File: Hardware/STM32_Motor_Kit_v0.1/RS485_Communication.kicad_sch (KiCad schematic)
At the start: 23 parts, among them J7 Conn_01x02_Male, U14 THVD1500D

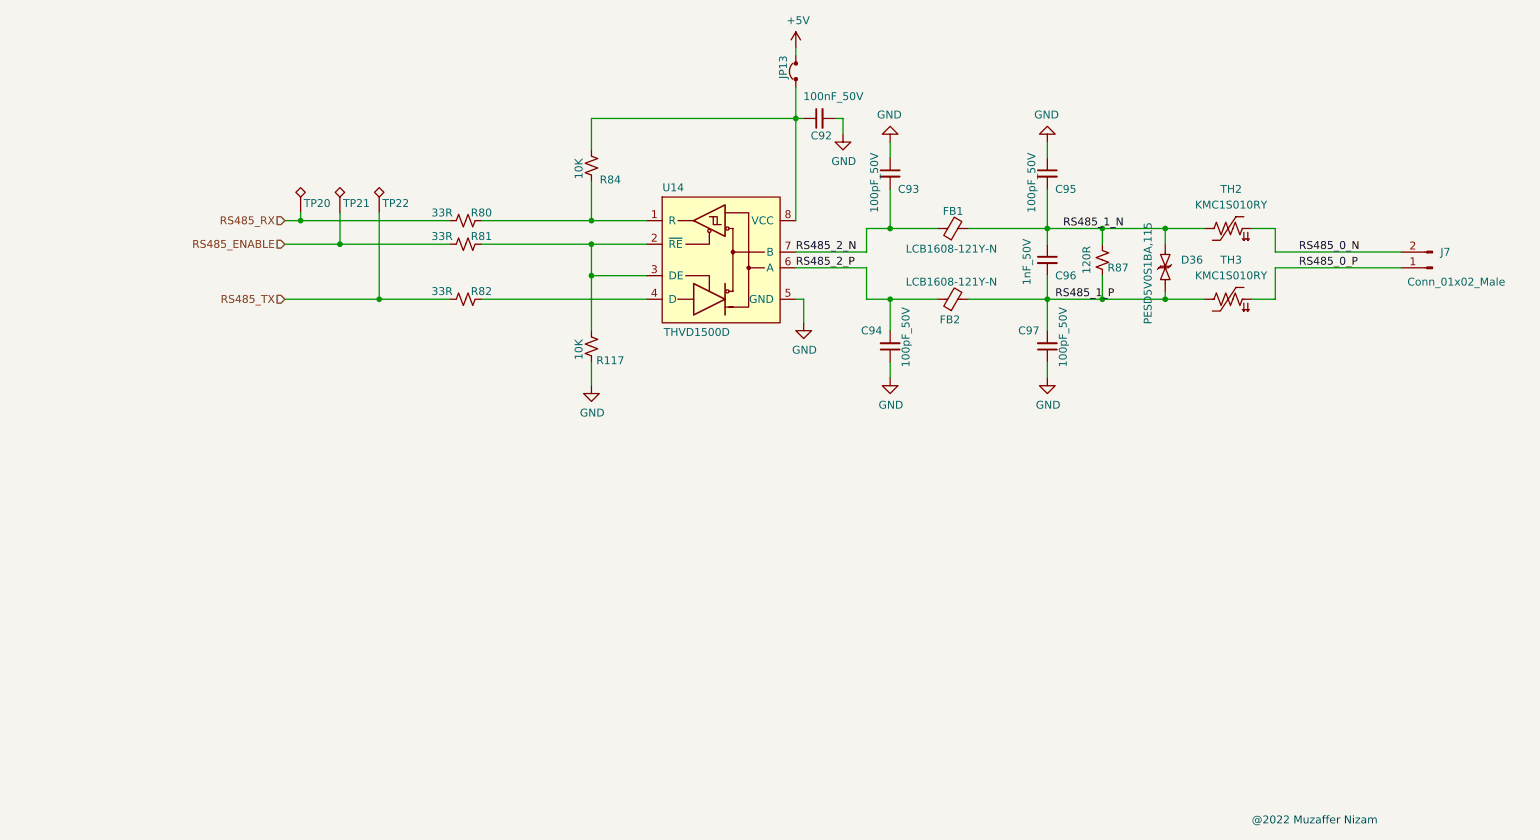
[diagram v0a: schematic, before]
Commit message: 12.01.2025
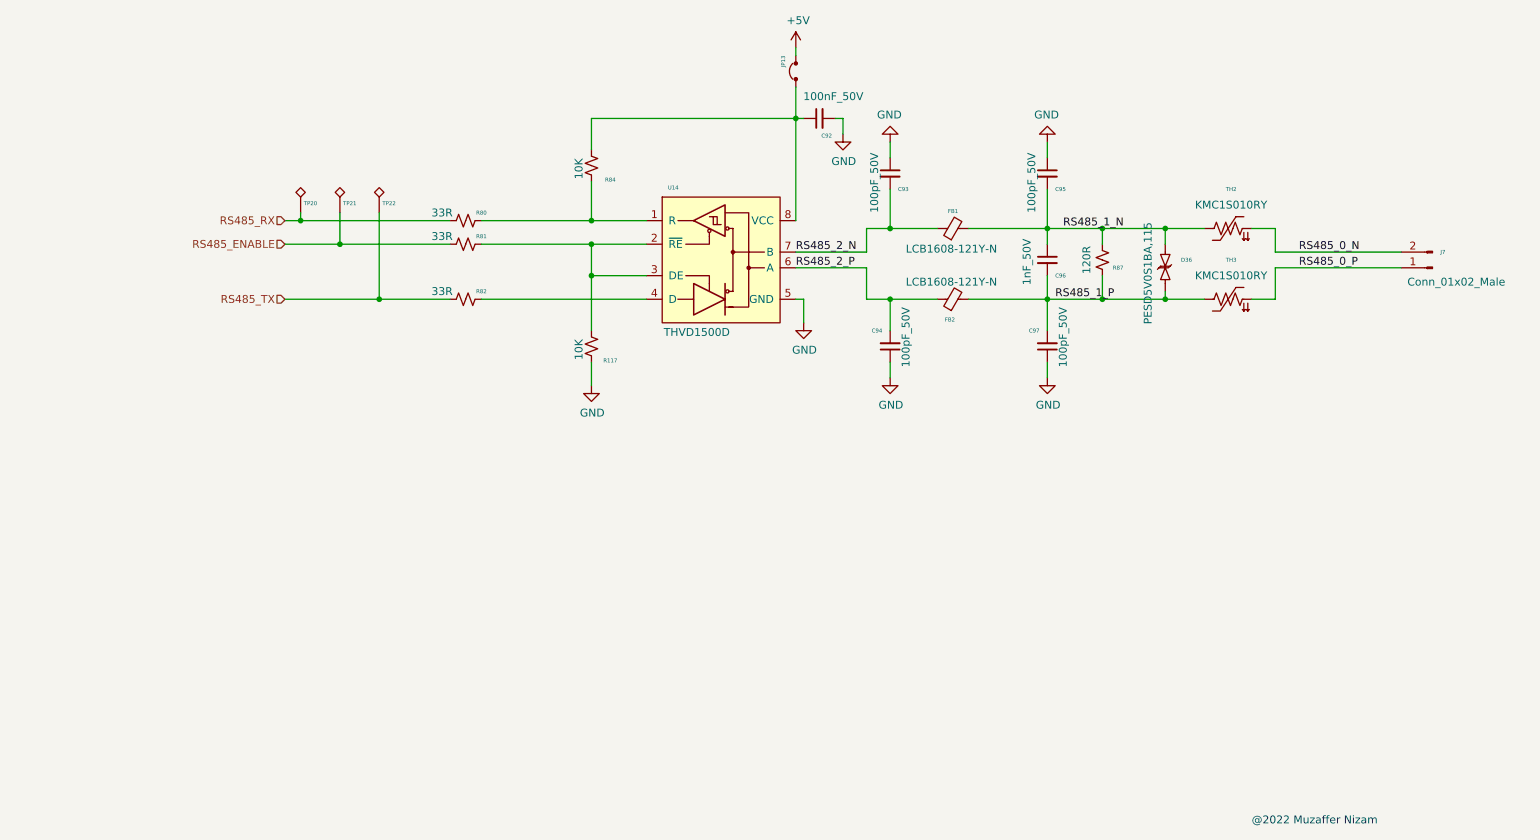
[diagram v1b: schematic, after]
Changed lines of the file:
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@@
 			(effects
 				(font
-					(size 1.27 1.27)
+					(face "Arial")
+					(size 0.635 0.635)
 				)
 			)
@@
 			(effects
 				(font
-					(size 1.27 1.27)
+					(face "Arial")
+					(size 0.635 0.635)
 				)
 				(justify left)
@@
 			(effects
 				(font
-					(size 1.27 1.27)
+					(face "Arial")
+					(size 0.635 0.635)
 				)
 			)
@@
 			(effects
 				(font
-					(size 1.27 1.27)
+					(face "Arial")
+					(size 0.635 0.635)
 				)
 				(justify right)
@@
 			(effects
 				(font
-					(size 1.27 1.27)
+					(face "Arial")
+					(size 0.635 0.635)
 				)
 				(justify left)
@@
 			(effects
 				(font
-					(size 1.27 1.27)
+					(face "Arial")
+					(size 0.635 0.635)
 				)
 			)
@@
 			(effects
 				(font
-					(size 1.27 1.27)
+					(face "Arial")
+					(size 0.635 0.635)
 				)
 				(justify left)
@@
 			(effects
 				(font
-					(size 1.27 1.27)
+					(face "Arial")
+					(size 0.635 0.635)
 				)
 			)
@@
 			(effects
 				(font
-					(size 1.27 1.27)
+					(face "Arial")
+					(size 0.635 0.635)
 				)
 			)
@@
 			(effects
 				(font
-					(size 1.27 1.27)
+					(face "Arial")
+					(size 0.635 0.635)
 				)
 				(justify left)
@@
 			(effects
 				(font
-					(size 1.27 1.27)
+					(face "Arial")
+					(size 0.635 0.635)
 				)
 				(hide yes)
@@
 			(effects
 				(font
-					(size 1.27 1.27)
+					(face "Arial")
+					(size 0.635 0.635)
 				)
 				(hide yes)
@@
 			(effects
 				(font
-					(size 1.27 1.27)
+					(face "Arial")
+					(size 0.635 0.635)
 				)
 				(justify left)
@@
 			(effects
 				(font
-					(size 1.27 1.27)
+					(face "Arial")
+					(size 0.635 0.635)
 				)
 			)
@@
 			(effects
 				(font
-					(size 1.27 1.27)
+					(face "Arial")
+					(size 0.635 0.635)
 				)
 				(justify right)
@@
 			(effects
 				(font
-					(size 1.27 1.27)
+					(face "Arial")
+					(size 0.635 0.635)
 				)
 				(hide yes)
@@
 			(effects
 				(font
-					(size 1.27 1.27)
+					(face "Arial")
+					(size 0.635 0.635)
 				)
 				(hide yes)
@@
 			(effects
 				(font
-					(size 1.27 1.27)
+					(face "Arial")
+					(size 0.635 0.635)
 				)
 			)
@@
 			(effects
 				(font
-					(size 1.27 1.27)
+					(face "Arial")
+					(size 0.635 0.635)
 				)
 				(hide yes)
@@
 			(effects
 				(font
-					(size 1.27 1.27)
+					(face "Arial")
+					(size 0.635 0.635)
 				)
 				(hide yes)
@@
 			(effects
 				(font
-					(size 1.27 1.27)
+					(face "Arial")
+					(size 0.635 0.635)
 				)
 			)
@@
 			(effects
 				(font
-					(size 1.27 1.27)
+					(face "Arial")
+					(size 0.635 0.635)
 				)
 				(justify left)
@@
 			(effects
 				(font
-					(size 1.27 1.27)
+					(face "Arial")
+					(size 0.635 0.635)
 				)
 				(justify right)
@@
 			(effects
 				(font
-					(size 1.27 1.27)
+					(face "Arial")
+					(size 0.635 0.635)
 				)
 				(justify left)
@@
 			(effects
 				(font
-					(size 1.27 1.27)
+					(face "Arial")
+					(size 0.635 0.635)
 				)
 				(justify left)
@@
 			(effects
 				(font
-					(size 1.27 1.27)
+					(face "Arial")
+					(size 0.635 0.635)
 				)
 				(hide yes)
@@
 			(effects
 				(font
-					(size 1.27 1.27)
+					(face "Arial")
+					(size 0.635 0.635)
 				)
 			)
@@
 			(effects
 				(font
-					(size 1.27 1.27)
+					(face "Arial")
+					(size 0.635 0.635)
 				)
 				(hide yes)
@@
 			(effects
 				(font
-					(size 1.27 1.27)
+					(face "Arial")
+					(size 0.635 0.635)
 				)
 			)
@@
 			(effects
 				(font
-					(size 1.27 1.27)
+					(face "Arial")
+					(size 0.635 0.635)
 				)
 			)
@@
 			(effects
 				(font
-					(size 1.27 1.27)
+					(face "Arial")
+					(size 0.635 0.635)
 				)
 				(justify left)

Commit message: Şema üzerinde değişiklikler devam ediyor
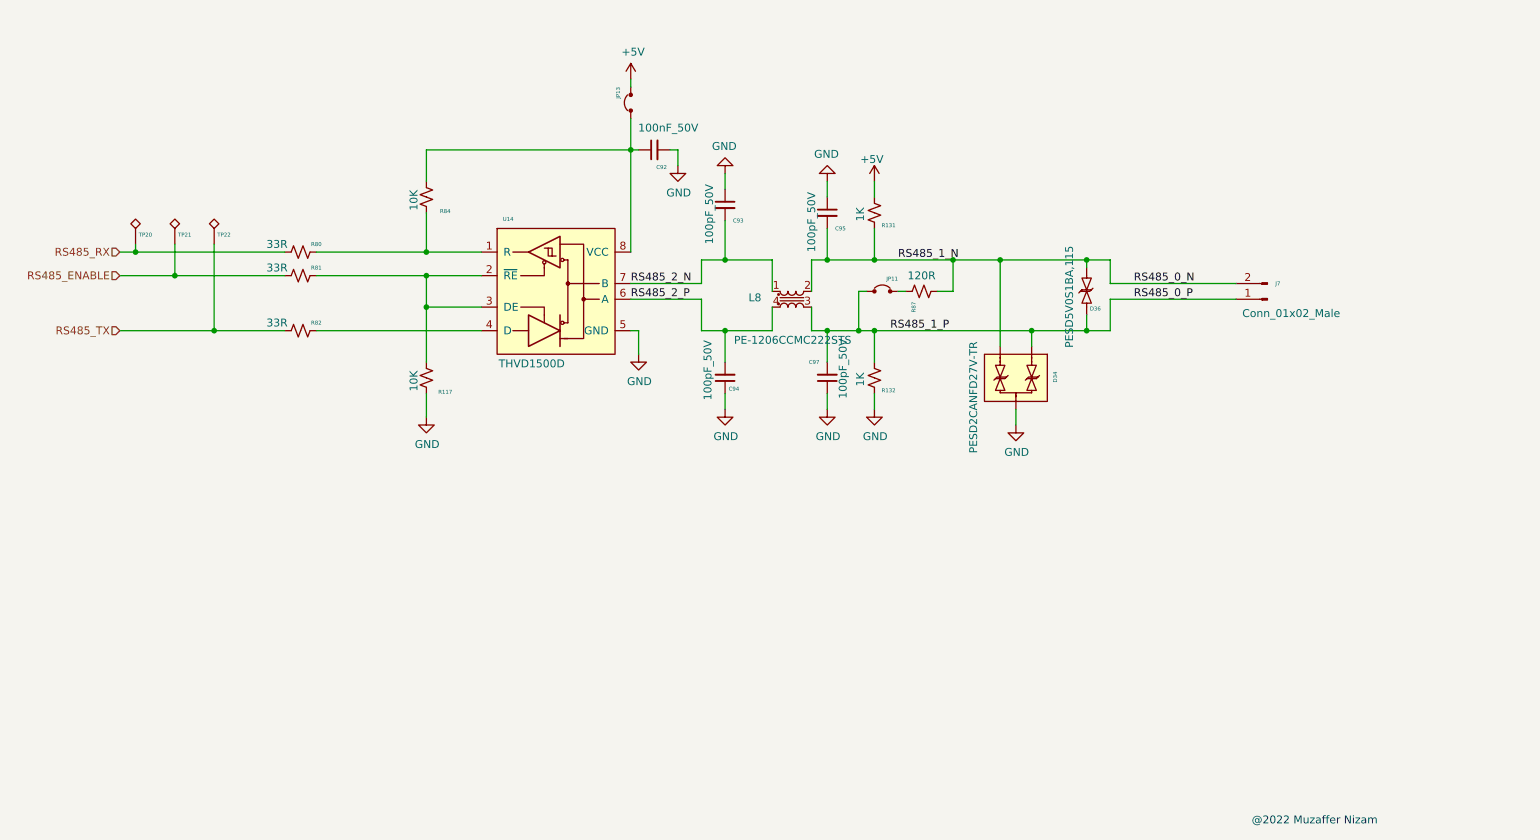
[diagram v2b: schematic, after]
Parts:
- removed C96: 1nF_50V, AKE_Capacitor_SMD:CAP_0603, symbol AKE_Capacitor:Capacitor_UnPolarised
- removed FB1, FB2: LCB1608-121Y-N, AKE_Resistor_SMD:RES_0603, symbol AKE_Inductor:Ferrite_Bead
- removed TH2, TH3: KMC1S010RY, AKE_Resistor_SMD:RES_0603, symbol AKE_NTC_PTC:PTC_Thermistor_US
- added D34: PESD2CANFD27V-TR, AKE_Diode_SMD:SOT-23, symbol DC_DCU_v0.1-rescue:PESD2CANFD27V-TR-AKE_Diode
- added JP11: Jumper_Pinheader, AKE_Pinheader_TH:PinHeader_1x02_P2.54mm_Vertical, symbol AKE_Device:Jumper_Pinheader
- added L8: PE-1206CCMC222STS, MN_Inductor_SMD:CMC_1206_4_LEAD, symbol MN_Inductor:PE-1206CCMC222STS
- added R131, R132: 1K, AKE_Resistor_SMD:RES_0603, symbol AKE_Resistor:Resistor_US
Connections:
- net RS485_1_N is gone; now on net RS485_0_N: C95.2, D36.2, R87.2
- net +5V: now also R131.2
- net GND: now also D34.3, R132.1
- net RS485_0_N: now also D34.2, L8.2, R131.1
- net RS485_0_P: now also C97.2, D36.1, D34.1, JP11.1 (A), L8.3, R132.2
- net RS485_2_N: now also L8.1
- net RS485_2_P: now also L8.4
- removed net RS485_1_P: C97.2, D36.1, R87.1
- new net: JP11.2 (B), R87.1
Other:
- moved on the sheet: C92, C93, C94, C95, C97, D36, J7, JP13, R117, R80, R81, R82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
